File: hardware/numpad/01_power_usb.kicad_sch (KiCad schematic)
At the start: 7 parts, among them J1 USB_C_Receptacle_USB2.0_16P, U1 NCP1117-3.3_SOT223, U2 USBLC6-2SC6

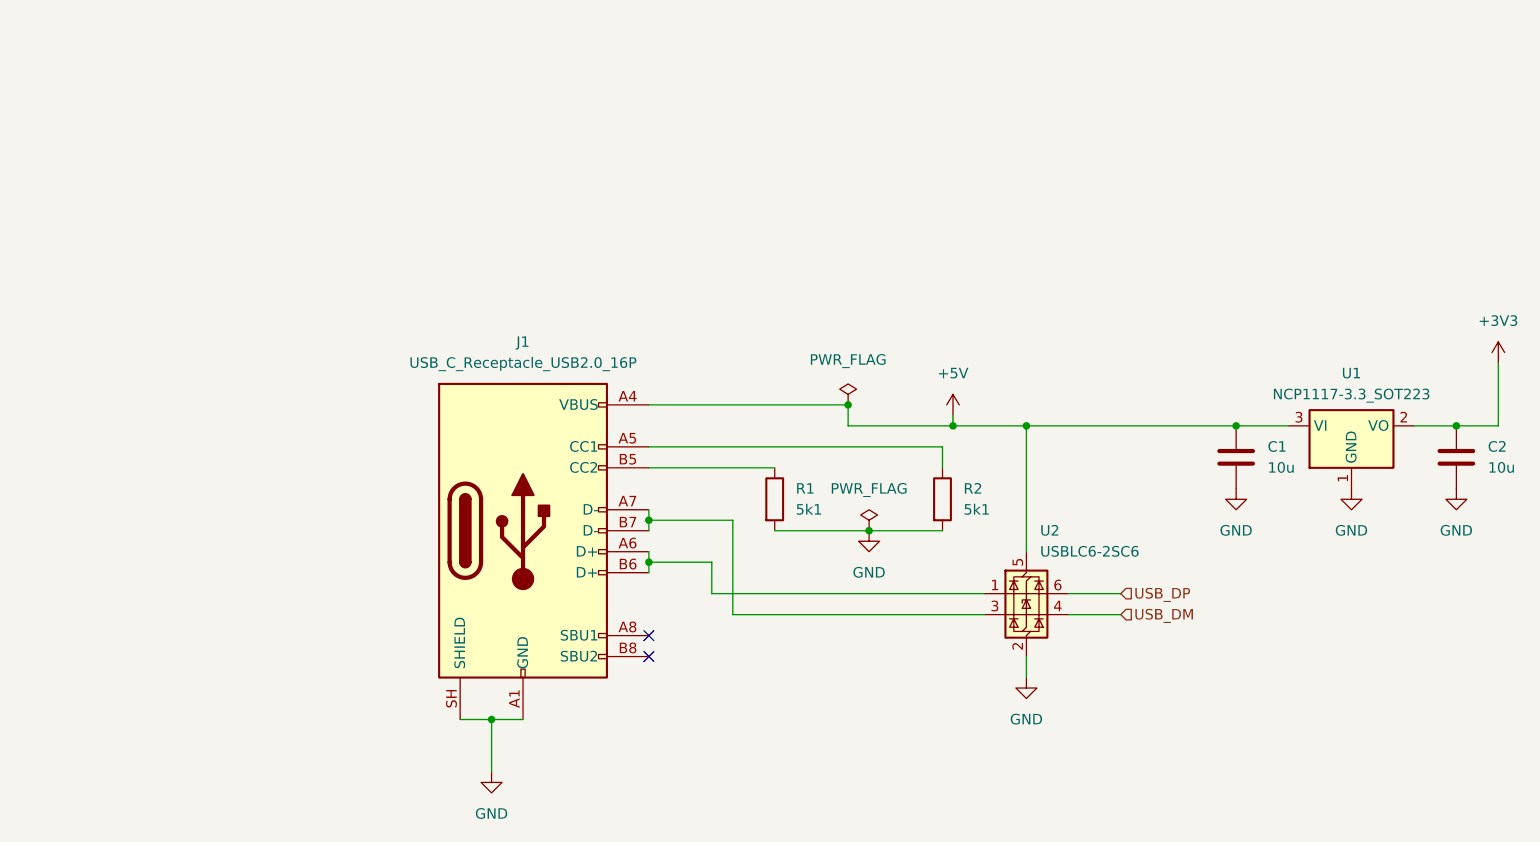
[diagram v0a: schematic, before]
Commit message: Format cleanup, titles
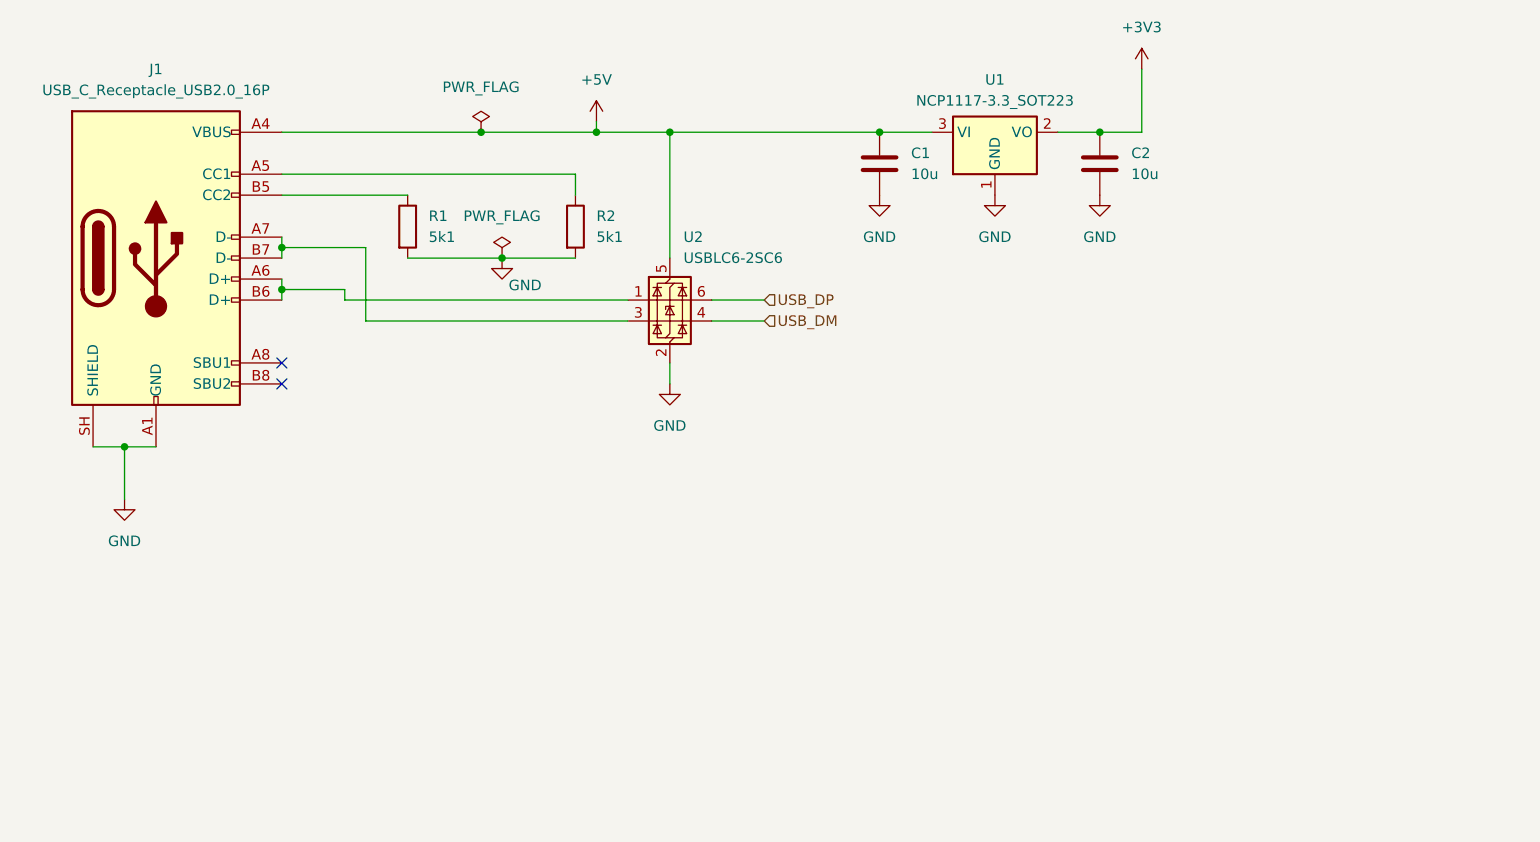
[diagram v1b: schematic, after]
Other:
- title: (none) -> Power and USB-C
- moved on the sheet: C1, C2, J1, R1, R2, U1, U2

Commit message: footprints set
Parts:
- C1, C2: footprint (none) -> Capacitor_SMD:C_0805_2012Metric
- J1: footprint (none) -> Connector_USB:USB_C_Receptacle_HRO_TYPE-C-31-M-12
- R1, R2: footprint (none) -> Resistor_SMD:R_0603_1608Metric
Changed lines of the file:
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@@
 			)
 		)
-		(property "Footprint" ""
+		(property "Footprint" "Resistor_SMD:R_0603_1608Metric"
 			(at 80.772 59.69 90)
 			(hide yes)
@@
 			)
 		)
-		(property "Footprint" ""
+		(property "Footprint" "Capacitor_SMD:C_0805_2012Metric"
 			(at 167.3352 55.88 0)
 			(hide yes)
@@
 			)
 		)
-		(property "Footprint" ""
+		(property "Footprint" "Resistor_SMD:R_0603_1608Metric"
 			(at 101.092 59.69 90)
 			(hide yes)
@@
 			)
 		)
-		(property "Footprint" ""
+		(property "Footprint" "Connector_USB:USB_C_Receptacle_HRO_TYPE-C-31-M-12"
 			(at 55.88 63.5 0)
 			(hide yes)
@@
 			)
 		)
-		(property "Footprint" ""
+		(property "Footprint" "Capacitor_SMD:C_0805_2012Metric"
 			(at 140.6652 55.88 0)
 			(hide yes)
